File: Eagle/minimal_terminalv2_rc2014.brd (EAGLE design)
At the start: 102.7 x 65 mm, 30 parts, among them IC1 7806T, IC2 74HC166N, X1 VGA Output

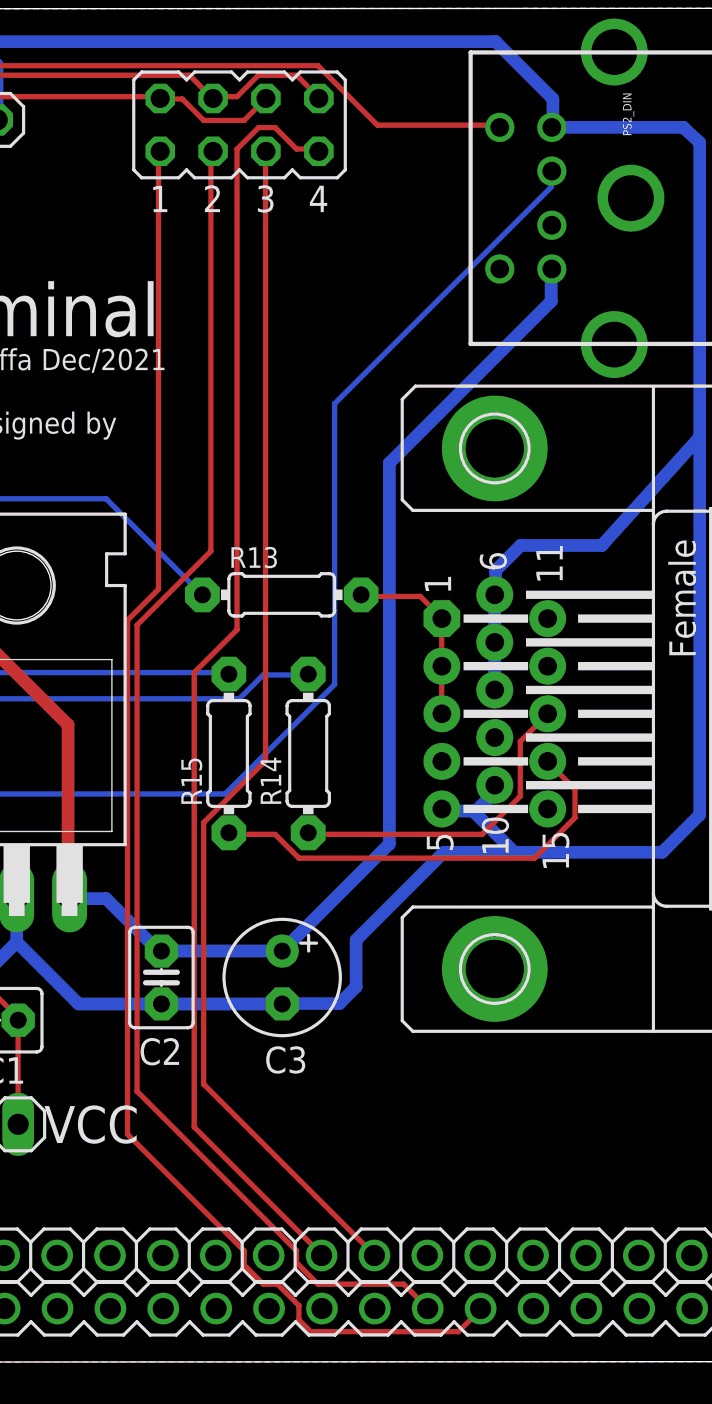
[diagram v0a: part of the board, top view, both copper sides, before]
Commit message: .  updating eagle files with last fixes.
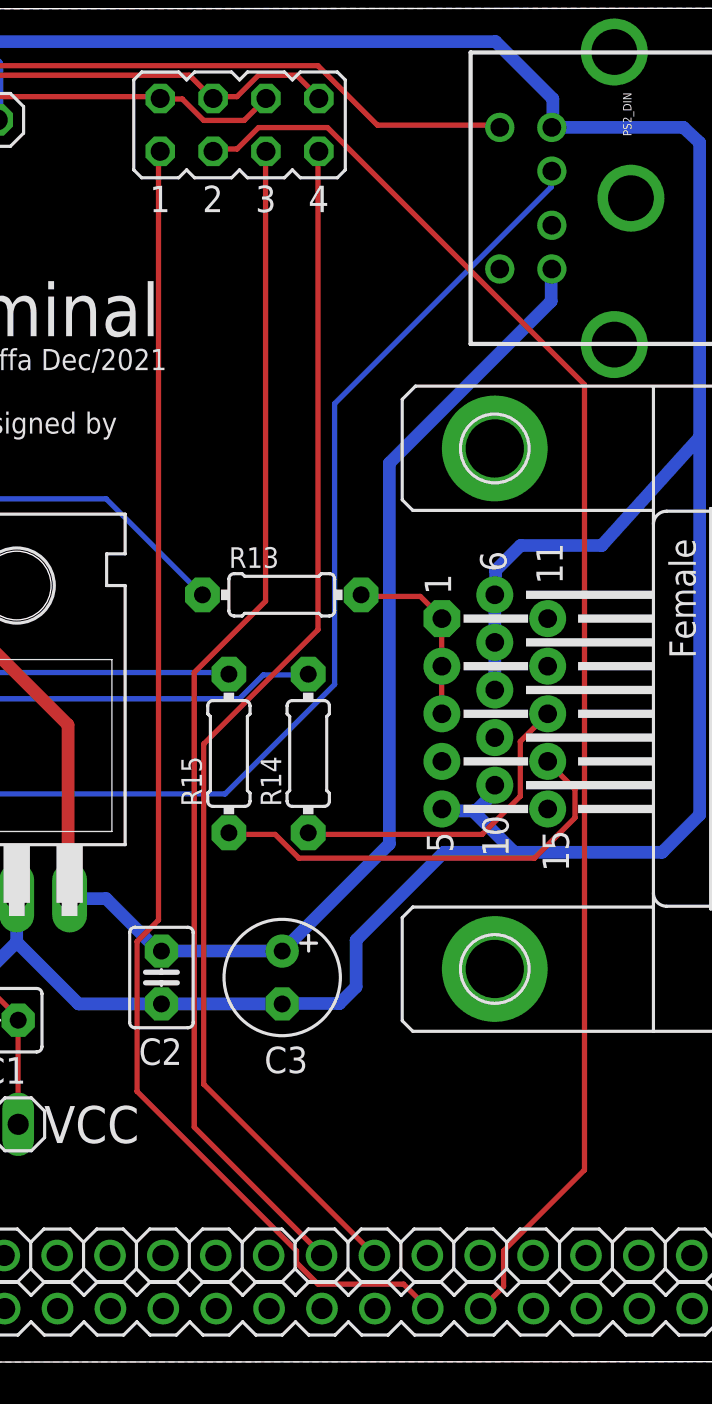
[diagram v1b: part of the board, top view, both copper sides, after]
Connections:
- net RXA: now also JP2.3; no longer JP2.1
- net RXB: now also JP2.7; no longer JP2.5
- net TXA: now also JP2.1; no longer JP2.3
- net TXB: now also JP2.5; no longer JP2.7
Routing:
- net TXB: track 61.4 -> 57.0 mm
- net TXA: track 65.3 -> 64.3 mm
- net RXB: track 57.7 -> 58.7 mm
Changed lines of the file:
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@@
 <signal name="RXA">
 <contactref element="JP3" pad="36"/>
-<contactref element="JP2" pad="1"/>
-<wire x1="75.2094" y1="37.1475" x2="75.2094" y2="58.1787" width="0.254" layer="1"/>
-<wire x1="73.7235" y1="35.6616" x2="75.2094" y2="37.1475" width="0.254" layer="1"/>
-<wire x1="73.7235" y1="10.9728" x2="73.7235" y2="35.6616" width="0.254" layer="1"/>
-<wire x1="79.3242" y1="5.3721" x2="73.7235" y2="10.9728" width="0.254" layer="1"/>
-<wire x1="79.3242" y1="4.6863" x2="79.3242" y2="5.3721" width="0.254" layer="1"/>
-<wire x1="80.2386" y1="3.7719" x2="79.3242" y2="4.6863" width="0.254" layer="1"/>
-<wire x1="80.9244" y1="3.7719" x2="80.2386" y2="3.7719" width="0.254" layer="1"/>
-<wire x1="81.9531" y1="2.7432" x2="80.9244" y2="3.7719" width="0.254" layer="1"/>
-<wire x1="81.9531" y1="2.0574" x2="81.9531" y2="2.7432" width="0.254" layer="1"/>
-<wire x1="82.5246" y1="1.4859" x2="81.9531" y2="2.0574" width="0.254" layer="1"/>
-<wire x1="89.6112" y1="1.4859" x2="82.5246" y2="1.4859" width="0.254" layer="1"/>
-<wire x1="90.6399" y1="2.5146" x2="89.6112" y2="1.4859" width="0.254" layer="1"/>
-<wire x1="75.2094" y1="58.1787" x2="75.29" y2="58.18" width="0.254" layer="1"/>
-<wire x1="90.6399" y1="2.5146" x2="90.68" y2="2.6" width="0.254" layer="1"/>
+<contactref element="JP2" pad="3"/>
+<wire x1="78.9813" y1="58.293" x2="77.8383" y2="58.293" width="0.254" layer="1"/>
+<wire x1="80.01" y1="59.3217" x2="78.9813" y2="58.293" width="0.254" layer="1"/>
+<wire x1="83.3247" y1="59.3217" x2="80.01" y2="59.3217" width="0.254" layer="1"/>
+<wire x1="95.6691" y1="46.9773" x2="83.3247" y2="59.3217" width="0.254" layer="1"/>
+<wire x1="95.6691" y1="9.2583" x2="95.6691" y2="46.9773" width="0.254" layer="1"/>
+<wire x1="91.7829" y1="5.3721" x2="95.6691" y2="9.2583" width="0.254" layer="1"/>
+<wire x1="91.7829" y1="3.6576" x2="91.7829" y2="5.3721" width="0.254" layer="1"/>
+<wire x1="90.7542" y1="2.6289" x2="91.7829" y2="3.6576" width="0.254" layer="1"/>
+<wire x1="77.8383" y1="58.293" x2="77.83" y2="58.18" width="0.254" layer="1"/>
+<wire x1="90.7542" y1="2.6289" x2="90.68" y2="2.6" width="0.254" layer="1"/>
 </signal>
 <signal name="TXA">
 <contactref element="JP3" pad="35"/>
-<contactref element="JP2" pad="3"/>
-<wire x1="77.724" y1="38.9763" x2="77.724" y2="58.1787" width="0.254" layer="1"/>
-<wire x1="74.1807" y1="35.433" x2="77.724" y2="38.9763" width="0.254" layer="1"/>
-<wire x1="74.1807" y1="13.0302" x2="74.1807" y2="35.433" width="0.254" layer="1"/>
+<contactref element="JP2" pad="1"/>
+<wire x1="75.2094" y1="21.2598" x2="75.2094" y2="58.1787" width="0.254" layer="1"/>
+<wire x1="74.1807" y1="20.2311" x2="75.2094" y2="21.2598" width="0.254" layer="1"/>
+<wire x1="74.1807" y1="13.0302" x2="74.1807" y2="20.2311" width="0.254" layer="1"/>
 <wire x1="81.8388" y1="5.3721" x2="74.1807" y2="13.0302" width="0.254" layer="1"/>
 <wire x1="81.8388" y1="4.8006" x2="81.8388" y2="5.3721" width="0.254" layer="1"/>
@@
 <wire x1="86.9823" y1="3.7719" x2="82.8675" y2="3.7719" width="0.254" layer="1"/>
 <wire x1="88.1253" y1="2.6289" x2="86.9823" y2="3.7719" width="0.254" layer="1"/>
-<wire x1="77.724" y1="58.1787" x2="77.83" y2="58.18" width="0.254" layer="1"/>
+<wire x1="75.2094" y1="58.1787" x2="75.29" y2="58.18" width="0.254" layer="1"/>
 <wire x1="88.1253" y1="2.6289" x2="88.14" y2="2.6" width="0.254" layer="1"/>
 </signal>
 <signal name="RXB">
 <contactref element="JP4" pad="18"/>
-<contactref element="JP2" pad="5"/>
-<wire x1="80.3529" y1="28.9179" x2="80.3529" y2="58.1787" width="0.254" layer="1"/>
-<wire x1="77.3811" y1="25.9461" x2="80.3529" y2="28.9179" width="0.254" layer="1"/>
-<wire x1="77.3811" y1="13.3731" x2="77.3811" y2="25.9461" width="0.254" layer="1"/>
+<contactref element="JP2" pad="7"/>
+<wire x1="82.8675" y1="35.2044" x2="82.8675" y2="58.1787" width="0.254" layer="1"/>
+<wire x1="77.3811" y1="29.718" x2="82.8675" y2="35.2044" width="0.254" layer="1"/>
+<wire x1="77.3811" y1="13.3731" x2="77.3811" y2="29.718" width="0.254" layer="1"/>
 <wire x1="85.4964" y1="5.2578" x2="77.3811" y2="13.3731" width="0.254" layer="1"/>
-<wire x1="80.3529" y1="58.1787" x2="80.37" y2="58.18" width="0.254" layer="1"/>
+<wire x1="82.8675" y1="58.1787" x2="82.91" y2="58.18" width="0.254" layer="1"/>
 <wire x1="85.4964" y1="5.2578" x2="85.58" y2="5.15" width="0.254" layer="1"/>
 </signal>
 <signal name="TXB">
 <contactref element="JP4" pad="17"/>
-<contactref element="JP2" pad="7"/>
-<wire x1="81.8388" y1="58.293" x2="82.8675" y2="58.293" width="0.254" layer="1"/>
-<wire x1="80.8101" y1="59.3217" x2="81.8388" y2="58.293" width="0.254" layer="1"/>
-<wire x1="80.01" y1="59.3217" x2="80.8101" y2="59.3217" width="0.254" layer="1"/>
-<wire x1="78.9813" y1="58.293" x2="80.01" y2="59.3217" width="0.254" layer="1"/>
-<wire x1="78.9813" y1="35.2044" x2="78.9813" y2="58.293" width="0.254" layer="1"/>
-<wire x1="76.9239" y1="33.147" x2="78.9813" y2="35.2044" width="0.254" layer="1"/>
+<contactref element="JP2" pad="5"/>
+<wire x1="80.3529" y1="36.576" x2="80.3529" y2="58.1787" width="0.254" layer="1"/>
+<wire x1="76.9239" y1="33.147" x2="80.3529" y2="36.576" width="0.254" layer="1"/>
 <wire x1="76.9239" y1="11.3157" x2="76.9239" y2="33.147" width="0.254" layer="1"/>
 <wire x1="82.9818" y1="5.2578" x2="76.9239" y2="11.3157" width="0.254" layer="1"/>
-<wire x1="82.8675" y1="58.293" x2="82.91" y2="58.18" width="0.254" layer="1"/>
+<wire x1="80.3529" y1="58.1787" x2="80.37" y2="58.18" width="0.254" layer="1"/>
 <wire x1="82.9818" y1="5.2578" x2="83.04" y2="5.15" width="0.254" layer="1"/>
 </signal>
